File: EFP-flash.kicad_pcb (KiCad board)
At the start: 2 copper layers, 30 x 18.4 mm, 17 parts, among them J101 USB_C_Receptacle_USB2.0, J102 Conn_01x06, Q101 MMDT3904, SW101 SW_SPDT, U101 ESD PROTECTION, U102 TLV75533PDBV, U103 CH340C

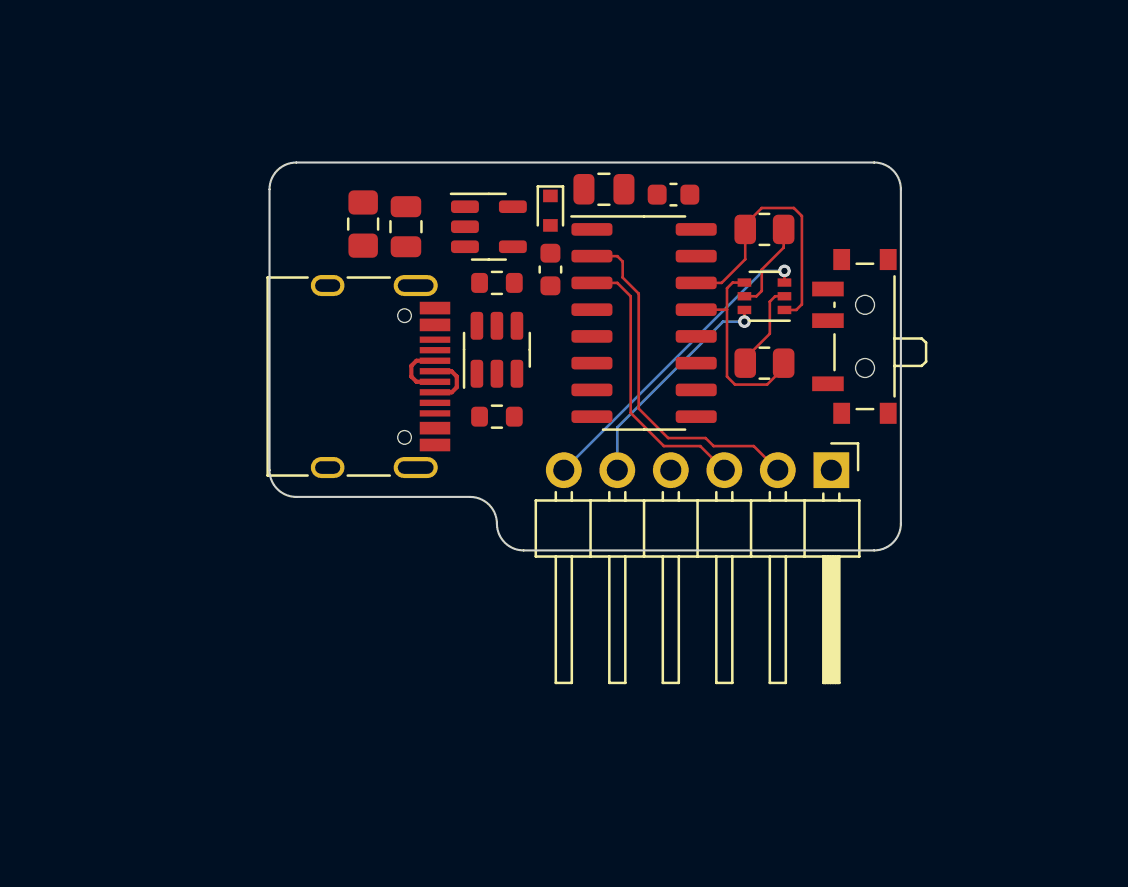
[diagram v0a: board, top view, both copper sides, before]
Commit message: PCB complete
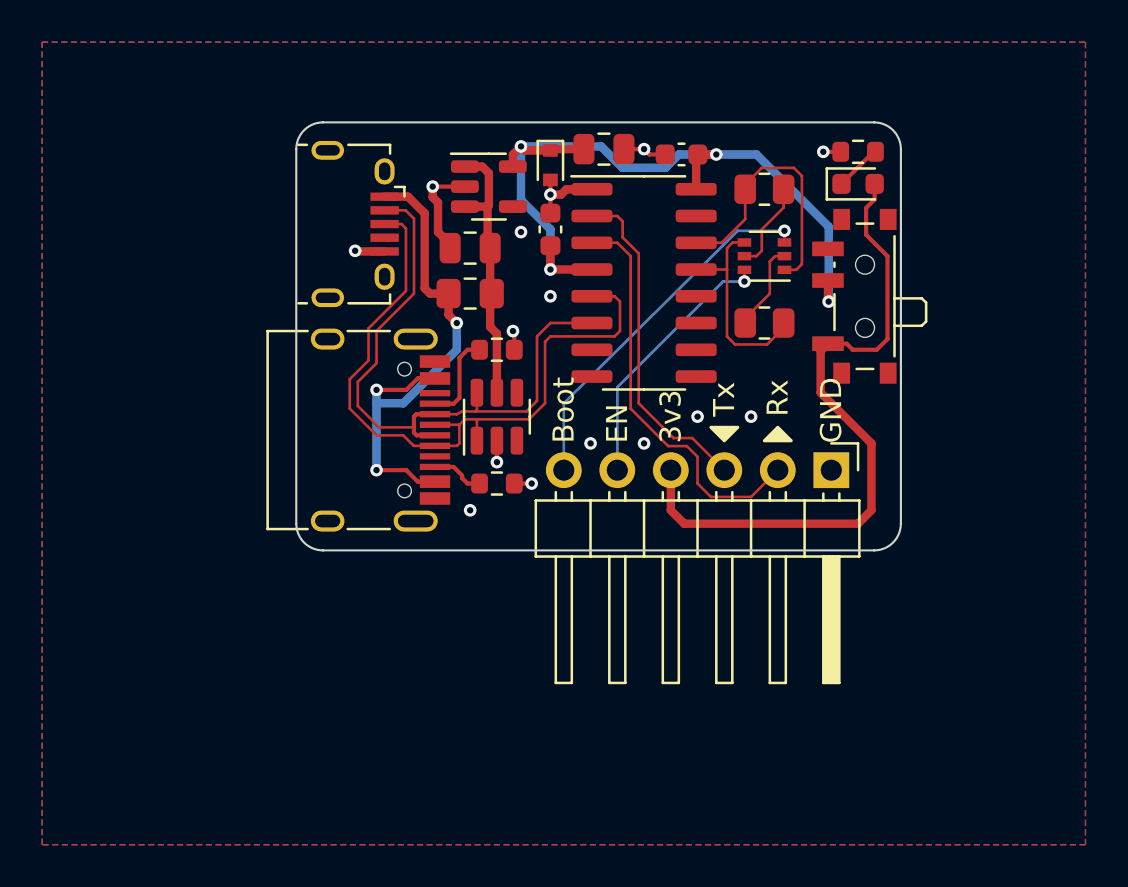
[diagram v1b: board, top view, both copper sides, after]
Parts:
- added D102: GREEN, LED_SMD:LED_0603_1608Metric, F.Cu at (151.1, 37.2)
- added J101: USB_B_Micro, Connector_USB_custom:USB_Micro-B_Amphenol_10118194_Horizontal, F.Cu at (127.3, 39.1)
- added LOGO101: Open_Hardware, Symbol:OSHW-Logo2_7.3x6mm_SilkScreen, B.Cu at (145.8, 42.5)
- added R105: 10kΩ, Resistor_SMD:R_0603_1608Metric, F.Cu at (151.1, 35.7)
- moved F101 6.06 mm to (132.7, 42.4), turned to 180 degrees
- moved C101 3.21 mm to (132.7, 40.3), turned to 180 degrees
- moved R101 3.18 mm to (134.0, 51.4)
- moved R102 3.18 mm to (134.0, 45.1)
- moved U101 3.17 mm to (134.0, 48.3)
- moved J102 2.54 mm to (127.0, 48.9)
- moved D101 2.16 mm to (136.5, 36.3)
- moved C104 1.94 mm to (142.7, 35.8)
- moved C102 1.91 mm to (139.1, 35.6)
- moved C103 1.91 mm to (136.5, 39.4)
- moved Q101 1.91 mm to (146.7, 40.6)
- moved R103 1.91 mm to (146.7, 43.8)
- moved SW101 1.91 mm to (151.1, 42.5)
- moved U102 1.91 mm to (133.6, 37.3)
- moved U103 1.91 mm to (141.0, 41.9)
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- renumbered J101 to J102, J102 to J103
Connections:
- J103 pad 2: /SER_TX -> /SER_RX
- J103 pad 3: /SER_RX -> /SER_TX
- U101 pad 1: /USB_D- -> /USB_D+
- U101 pad 6: /USB_D+ -> /USB_D-
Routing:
- net +3V3: track 0.00 -> 37.6 mm, vias 0 -> 4
- net /3v3_{SW}: track 0.00 -> 32.1 mm
- net /USB_D+: track 2.78 -> 33.8 mm
- net /USB_D-: track 2.96 -> 29.4 mm
- net Net-(F101-Pad2): track 0.00 -> 24.6 mm, vias 0 -> 3
- net GND: track 0.00 -> 15.5 mm, vias 0 -> 15
- net VBUS: track 0.00 -> 13.0 mm
- net /SER_RX: track 13.2 -> 19.3 mm
- net Net-(J102-PadA5): track 0.00 -> 4.29 mm
- net /Boot: track 14.9 -> 17.6 mm
- net Net-(J102-PadB5): track 0.00 -> 2.52 mm
- net Net-(D102-Pad1): track 0.00 -> 2.24 mm
- net /EN: track 10.7 -> 12.6 mm
- net /SER_TX: track 16.7 -> 15.9 mm
- added copper zone on B.Cu, net GND
- added copper zone on F.Cu, net GND
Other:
- board size 30 x 18.4 mm -> 28.7 x 20.3 mm
- board text added: "3v3"
- board text added: "Boot"
- board text added: "CP2102 USB->UART"
- board text added: "EN"
- board text added: "ESP-flash v1.0.0"
- board text added: "GND"
- board text added: "JLCJLCJLCJLC"
- board text added: "Rx"
- board text added: "Tx"
